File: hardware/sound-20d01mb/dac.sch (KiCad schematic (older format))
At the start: 13 parts

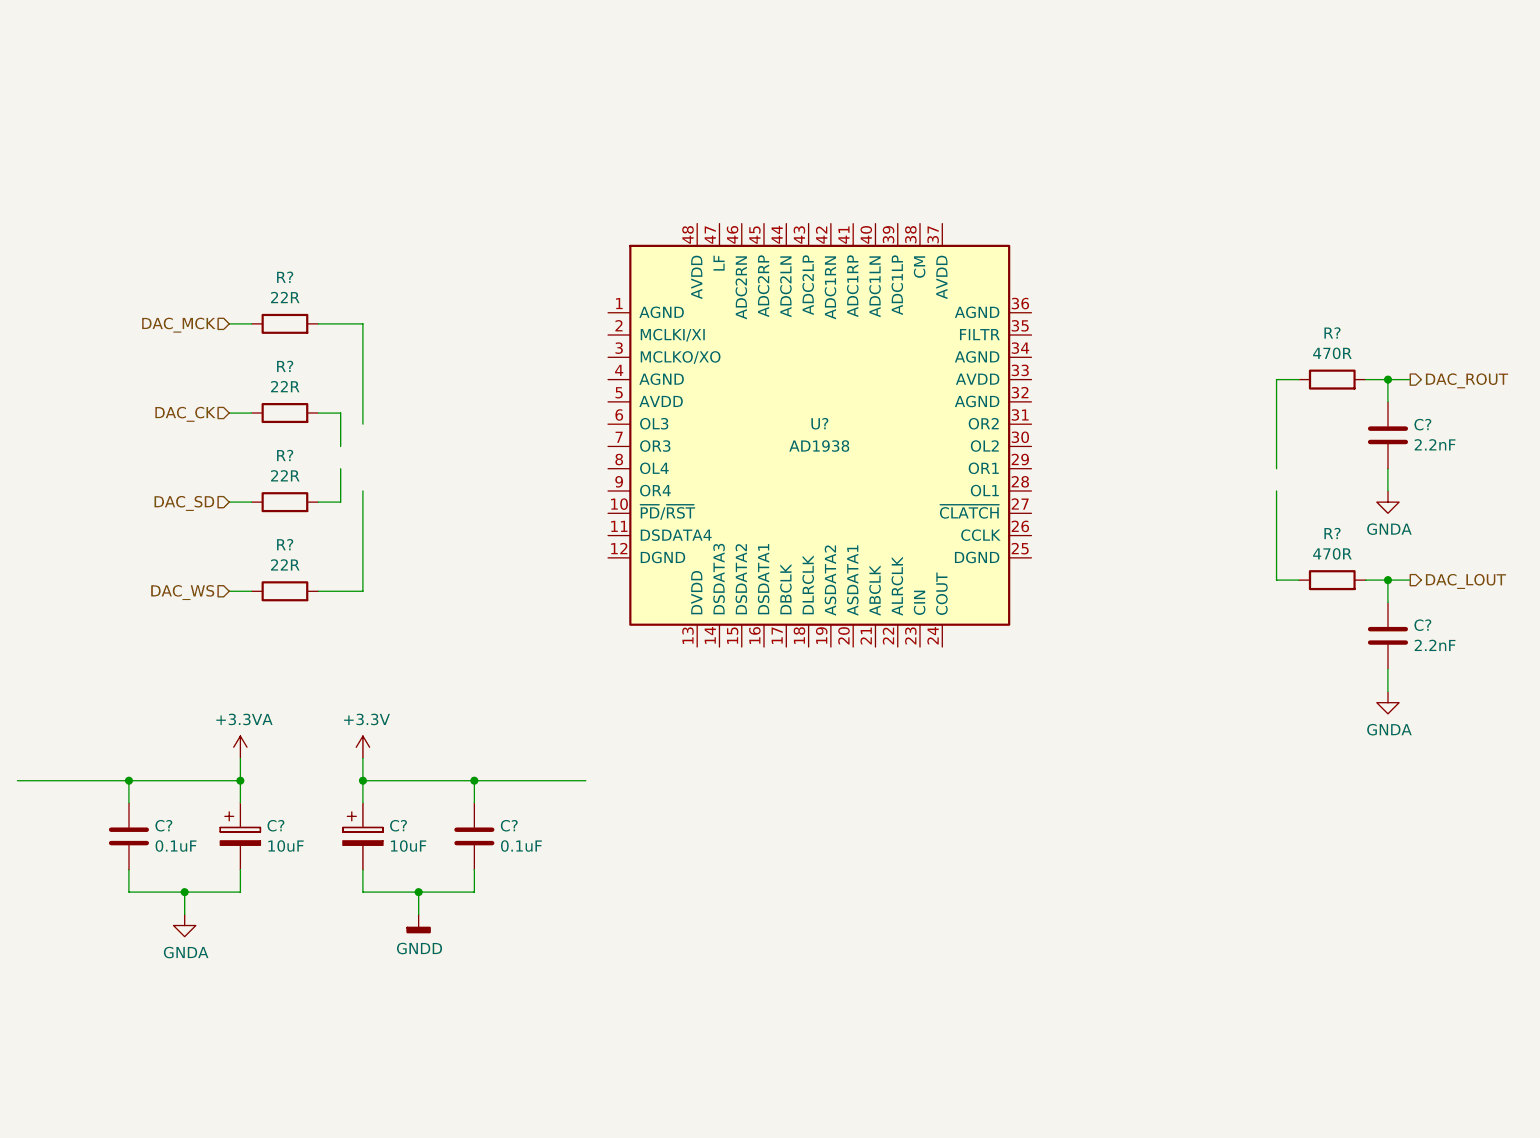
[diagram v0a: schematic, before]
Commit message: Updated schematics
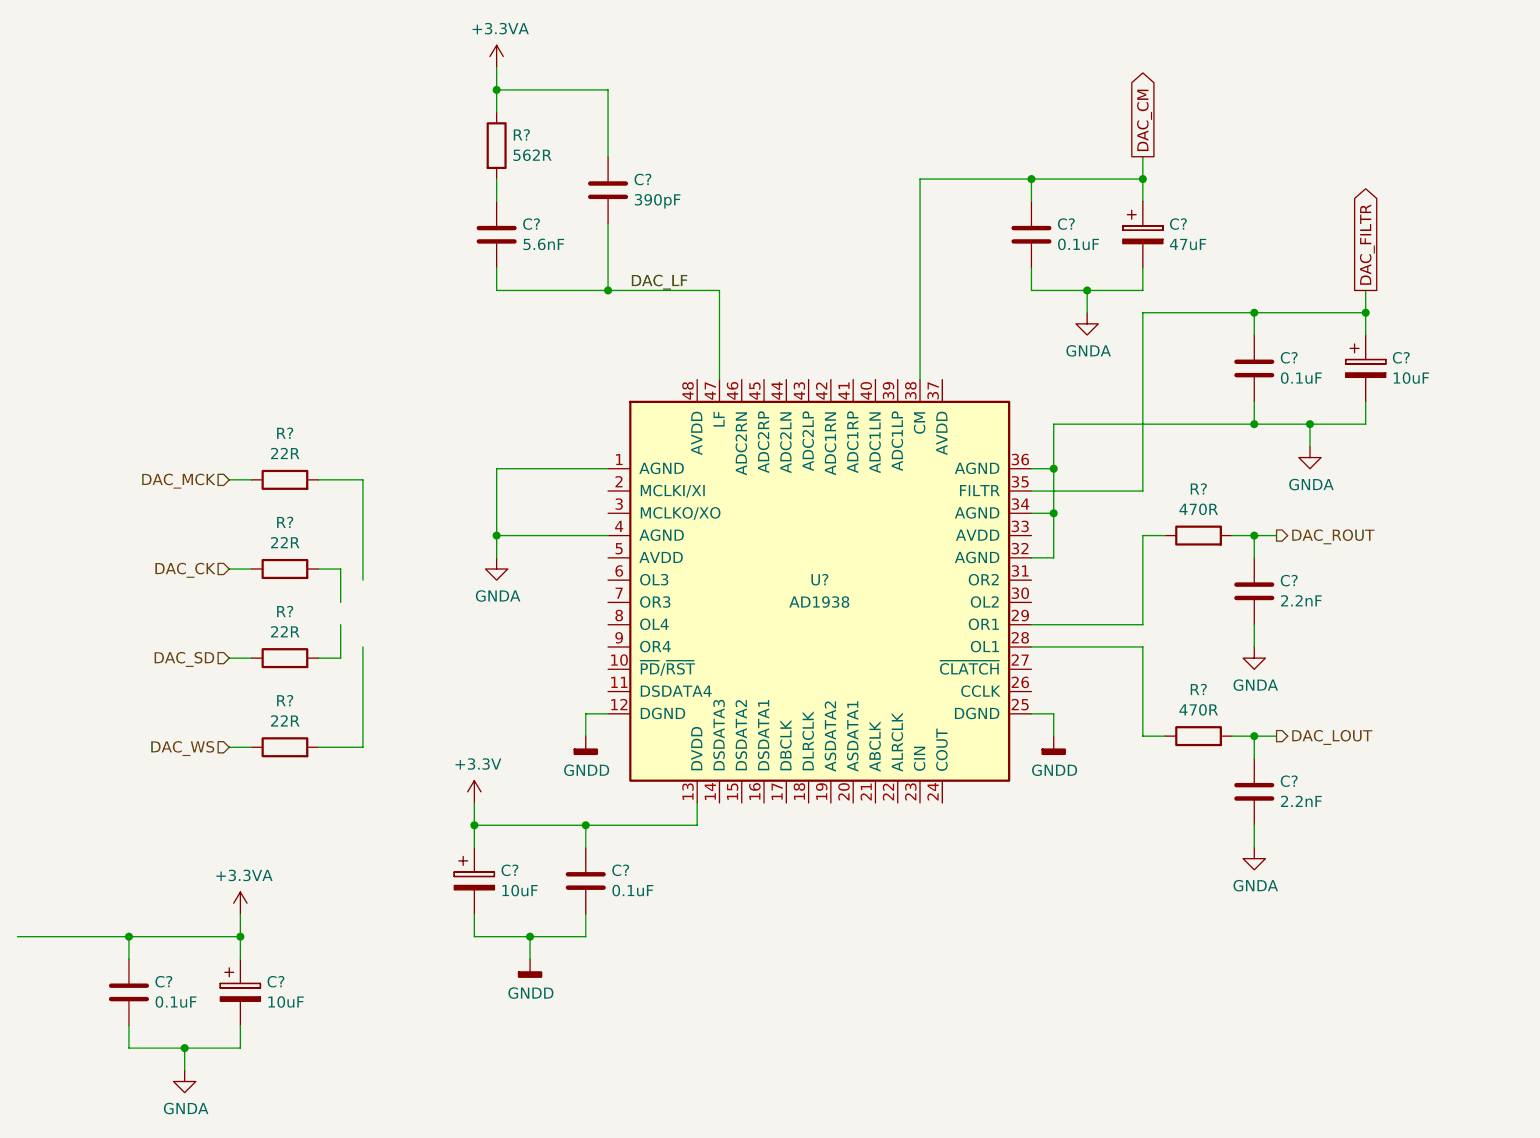
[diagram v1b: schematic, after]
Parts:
- added C?: 10uF, Capacitor_SMD:CP_Elec_4x5.4, symbol Device:CP
- added C? (x2): 0.1uF, Capacitor_SMD:C_1206_3216Metric_Pad1.42x1.75mm_HandSolder, symbol Device:C
- added C?: 47uF, symbol Device:CP
- added C?: 5.6nF, symbol Device:C
- added C?: 390pF, symbol Device:C
- added R?: 562R, symbol Device:R
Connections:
- net labels added: DAC_CM, DAC_FILTR, DAC_LF
- wire segments 44 -> 95
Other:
- moved on the sheet: C?, R?, U?
